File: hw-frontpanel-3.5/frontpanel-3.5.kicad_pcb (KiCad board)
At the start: 4 copper layers, 58.4 x 20.5 mm, 44 parts, among them J1 SPI, J2 QWIIC, J3 LED, J4 dbg, J5 OLED_SH1107, SW1 SW_Push, SW2 SW_Push, SW3 SW_Push, SW4 SW_Push, U1 MT3540, U2 LM809, U3 ESP32-C3-MINI-1

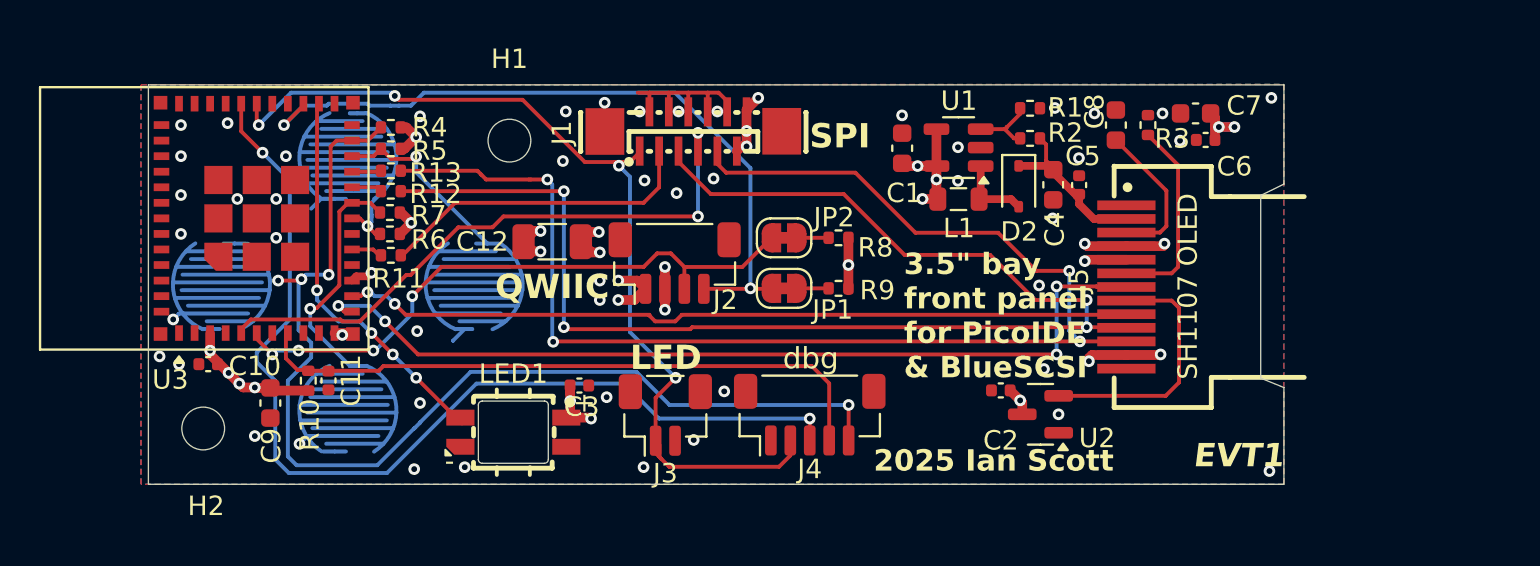
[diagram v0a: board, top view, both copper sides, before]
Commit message: Provisional v1.0.0 hardware
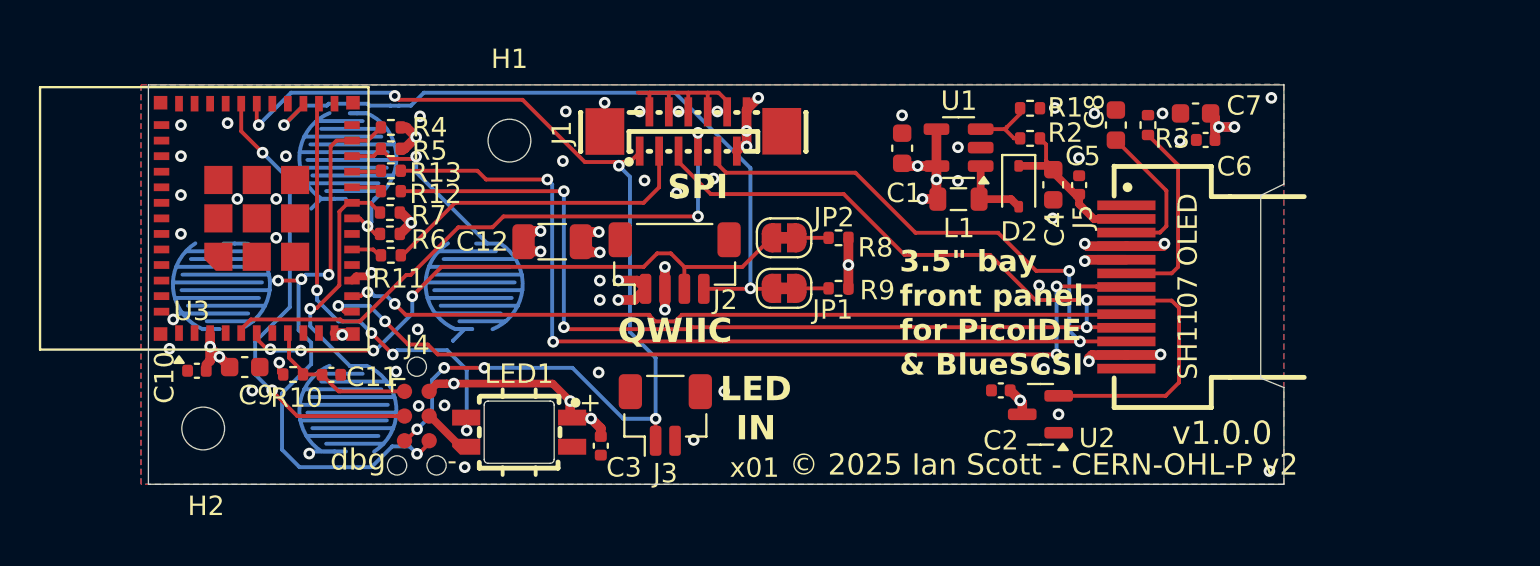
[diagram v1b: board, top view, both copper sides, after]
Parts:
- J4: value dbg -> TC2030; footprint Connector_JST:JST_SH_BM05B-SRSS-TB_1x05-1MP_P1.00mm_Vertical -> Connector:Tag-Connect_TC2030-IDC-NL_2x03_P1.27mm_Vertical
- moved J4 20.2 mm to (148.7, 58.8), turned to -90 degrees
- moved C3 3.29 mm to (158.2, 60.3), turned to -90 degrees
- moved C9 2.27 mm to (139.9, 56.2), turned to 0 degrees
- moved R10 0.84 mm to (142.4, 56.6), turned to 180 degrees
- moved C10 0.67 mm to (137.4, 56.4)
- moved C11 0.33 mm to (144.3, 56.6), turned to 0 degrees
- moved LED1 0.30 mm to (154.0, 59.6)
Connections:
- J4 pad 1: GND -> /ESP32_EN
- J4 pad 2: /ACT_LED_IN/UART_RX -> +3V3
- J4 pad 4: /ESP32_EN -> GND
- J4 pad 5: /P0_3 -> /ACT_LED_IN/UART_RX
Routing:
- net /UART_TX: track 52.2 -> 24.5 mm
- net /ESP32_EN: track 33.0 -> 8.05 mm
- net /P0_3: track 56.6 -> 31.9 mm
- net /ACT_LED_IN/UART_RX: track 48.5 -> 54.9 mm, vias 4 -> 7
- net +3V3: track 38.9 -> 45.0 mm
- net GND: track 26.7 -> 29.7 mm, vias 57 -> 56
- net /LED_DATA: track 20.8 -> 23.3 mm
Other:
- board text added: "LED IN"
- board text added: "v1.0.0"
- board text added: "x01"
- board text added: "© 2025 Ian Scott - CERN-OHL-P v2"
- board text removed: "2025 Ian Scott"
- board text removed: "EVT1"
- board text removed: "LED"
